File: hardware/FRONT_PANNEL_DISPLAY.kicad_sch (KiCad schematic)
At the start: 17 parts, among them SW1 SW_Push, SW2 SW_Push, U7 AS1115-BSST, U9 LTC-5723HR

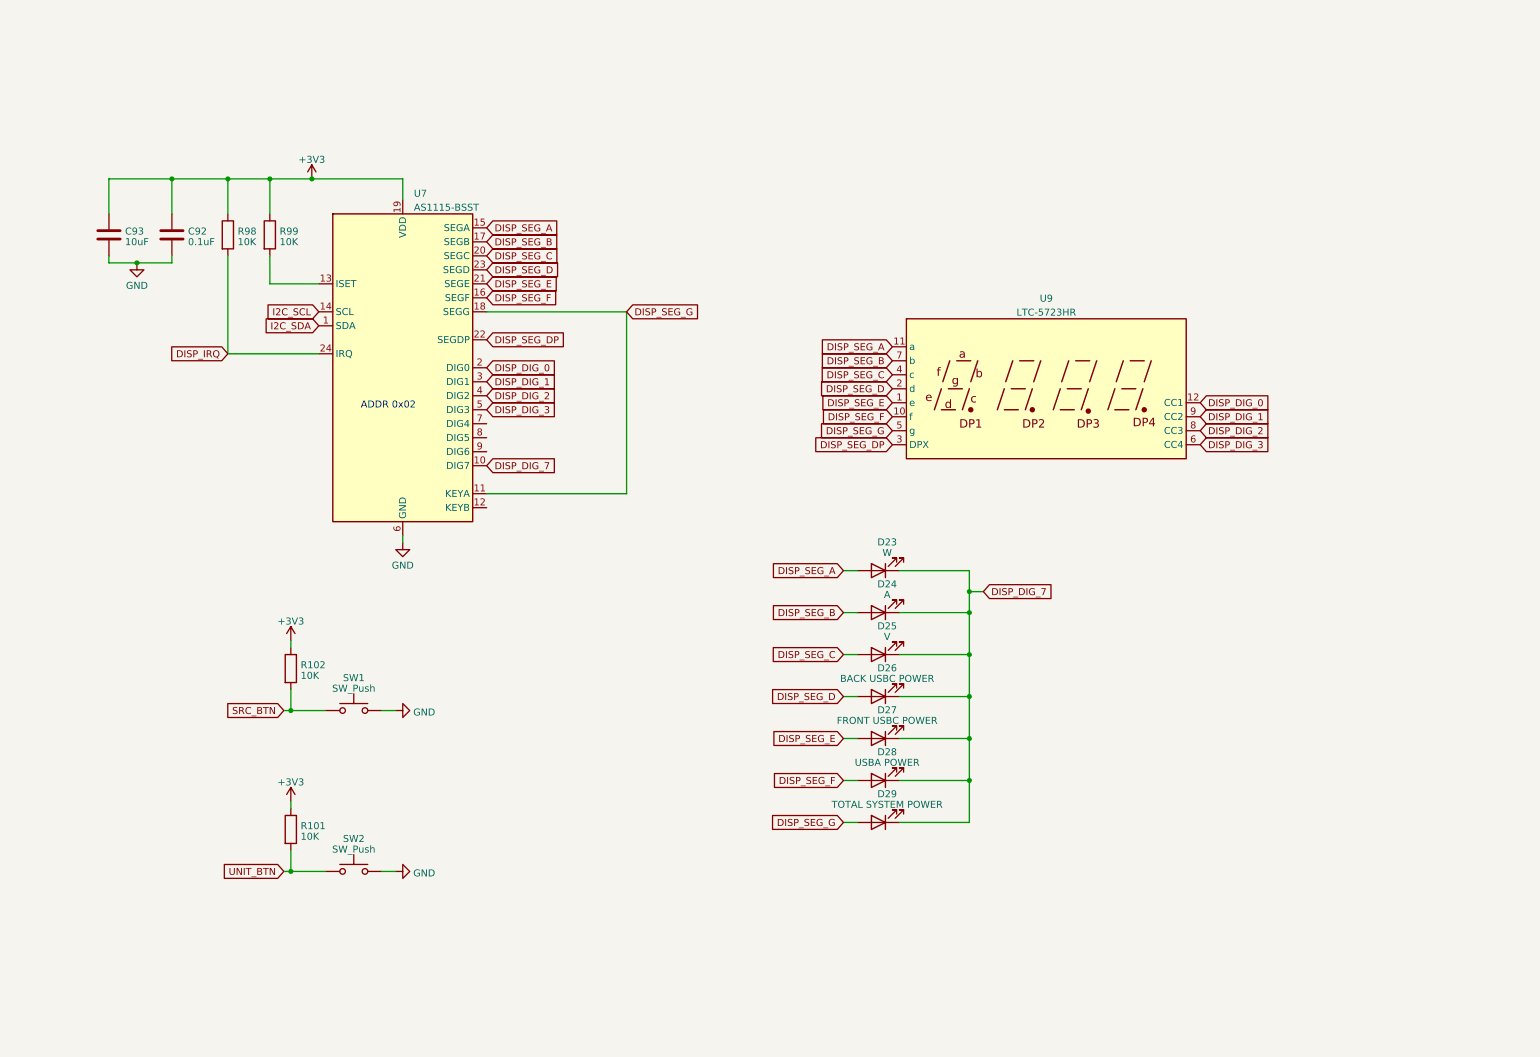
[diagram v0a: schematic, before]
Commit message: working on hardware
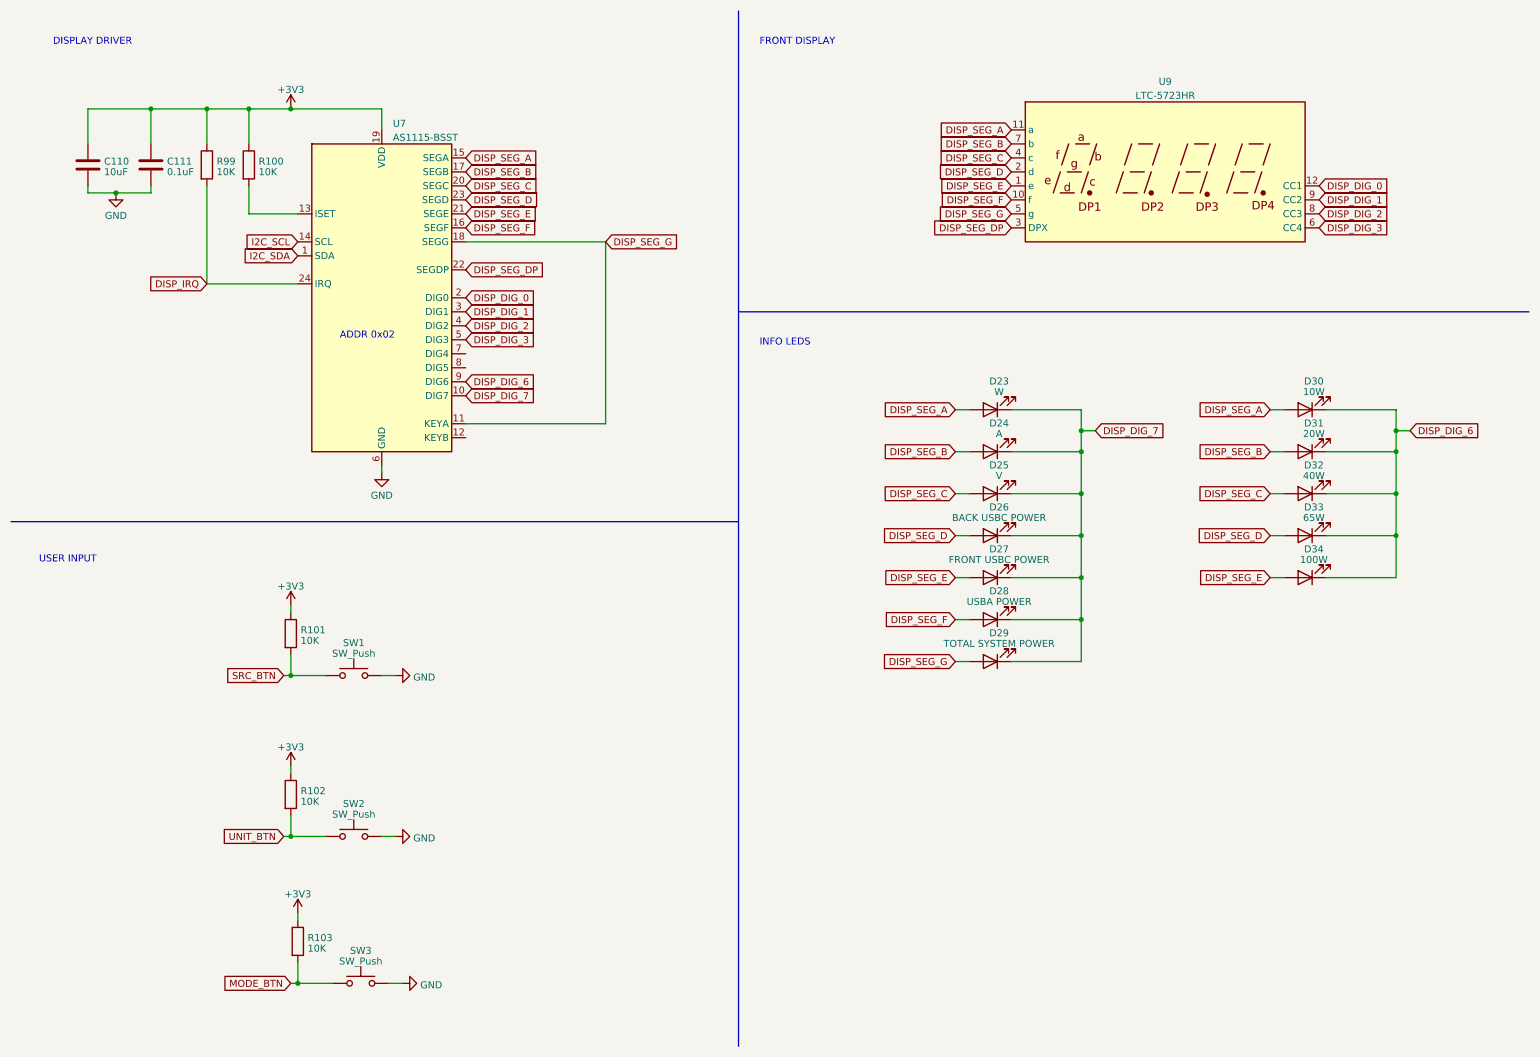
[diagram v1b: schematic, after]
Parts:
- added D30: 10W, Diode_SMD:D_0603_1608Metric, symbol Device:LED
- added D31: 20W, Diode_SMD:D_0603_1608Metric, symbol Device:LED
- added D32: 40W, Diode_SMD:D_0603_1608Metric, symbol Device:LED
- added D33: 65W, Diode_SMD:D_0603_1608Metric, symbol Device:LED
- added D34: 100W, Diode_SMD:D_0603_1608Metric, symbol Device:LED
- added R103: 10K, symbol Device:R
- added SW3: SW_Push, symbol Switch:SW_Push
- C110: renamed from C93; footprint (none) -> Capacitor_SMD:C_0603_1608Metric
- C111: renamed from C92; footprint (none) -> Capacitor_SMD:C_0603_1608Metric
- D23, D24, D25, D26, D27, D28, D29: footprint (none) -> Diode_SMD:D_0603_1608Metric
- renumbered R99 to R100, R102 to R101, R101 to R102, R98 to R99
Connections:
- net +3V3: now also R103.1
- net DISP_SEG_A: now also D30.2 (A)
- net DISP_SEG_B: now also D31.2 (A)
- net DISP_SEG_C: now also D32.2 (A)
- net DISP_SEG_D: now also D33.2 (A)
- net DISP_SEG_E: now also D34.2 (A)
- net GND: now also SW3.2
- net DISP_DIG_6: now reaches U7.9 (DIG6)
- net DISP_DIG_6: now also D30.1 (K), D31.1 (K), D32.1 (K), D33.1 (K), D34.1 (K)
- new net MODE_BTN: R103.2, SW3.1
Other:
- note added: "DISPLAY DRIVER"
- note added: "FRONT DISPLAY"
- note added: "INFO LEDS"
- note added: "USER INPUT"
- moved on the sheet: C110, C111, D23, D24, D25, D26, D27, D28, D29, R100, R101, R102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

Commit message: working assighning footprints still
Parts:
- R100, R101, R102, R103, R99: footprint (none) -> Resistor_SMD:R_0603_1608Metric
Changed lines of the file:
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@@
       (effects (font (size 1.27 1.27)) (justify left))
     )
-    (property "Footprint" "" (at 59.182 124.46 90)
+    (property "Footprint" "Resistor_SMD:R_0603_1608Metric" (at 59.182 124.46 90)
       (effects (font (size 1.27 1.27)) hide)
     )
@@
       (effects (font (size 1.27 1.27)) (justify left))
     )
-    (property "Footprint" "" (at 60.452 180.34 90)
+    (property "Footprint" "Resistor_SMD:R_0603_1608Metric" (at 60.452 180.34 90)
       (effects (font (size 1.27 1.27)) hide)
     )
@@
       (effects (font (size 1.27 1.27)) (justify left))
     )
-    (property "Footprint" "" (at 59.182 153.67 90)
+    (property "Footprint" "Resistor_SMD:R_0603_1608Metric" (at 59.182 153.67 90)
       (effects (font (size 1.27 1.27)) hide)
     )
@@
       (effects (font (size 1.27 1.27)) (justify left))
     )
-    (property "Footprint" "" (at 51.562 39.37 90)
+    (property "Footprint" "Resistor_SMD:R_0603_1608Metric" (at 51.562 39.37 90)
       (effects (font (size 1.27 1.27)) hide)
     )
@@
       (effects (font (size 1.27 1.27)) (justify left))
     )
-    (property "Footprint" "" (at 43.942 39.37 90)
-      (effects (font (size 1.27 1.27)) hide)
-    )
+    (property "Footprint" "Resistor_SMD:R_0603_1608Metric" (at 43.942 39.37 90)
+      (effects (font (size 1.27 1.27)) hide)
+    )

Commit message: FINALY starting the pcb
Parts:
- SW1, SW2, SW3: footprint (none) -> Button_Switch_THT:SW_PUSH_6mm
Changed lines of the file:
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@@
       (effects (font (size 1.27 1.27)))
     )
-    (property "Footprint" "" (at 73.66 182.88 0)
+    (property "Footprint" "Button_Switch_THT:SW_PUSH_6mm" (at 73.66 182.88 0)
       (effects (font (size 1.27 1.27)) hide)
     )
@@
       (effects (font (size 1.27 1.27)))
     )
-    (property "Footprint" "" (at 72.39 127 0)
+    (property "Footprint" "Button_Switch_THT:SW_PUSH_6mm" (at 72.39 127 0)
       (effects (font (size 1.27 1.27)) hide)
     )
@@
       (effects (font (size 1.27 1.27)))
     )
-    (property "Footprint" "" (at 72.39 156.21 0)
-      (effects (font (size 1.27 1.27)) hide)
-    )
+    (property "Footprint" "Button_Switch_THT:SW_PUSH_6mm" (at 72.39 156.21 0)
+      (effects (font (size 1.27 1.27)) hide)
+    )
